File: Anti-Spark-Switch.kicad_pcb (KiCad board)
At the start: 2 copper layers, 63.2 x 30 mm, 40 parts, among them P2 Pad_Conn, P5 Pad_Conn, P6 Pad_Conn, P7 CONN_01X04, Q1 IRFS7530, Q2 IRFS7530, Q3 IRFS7530

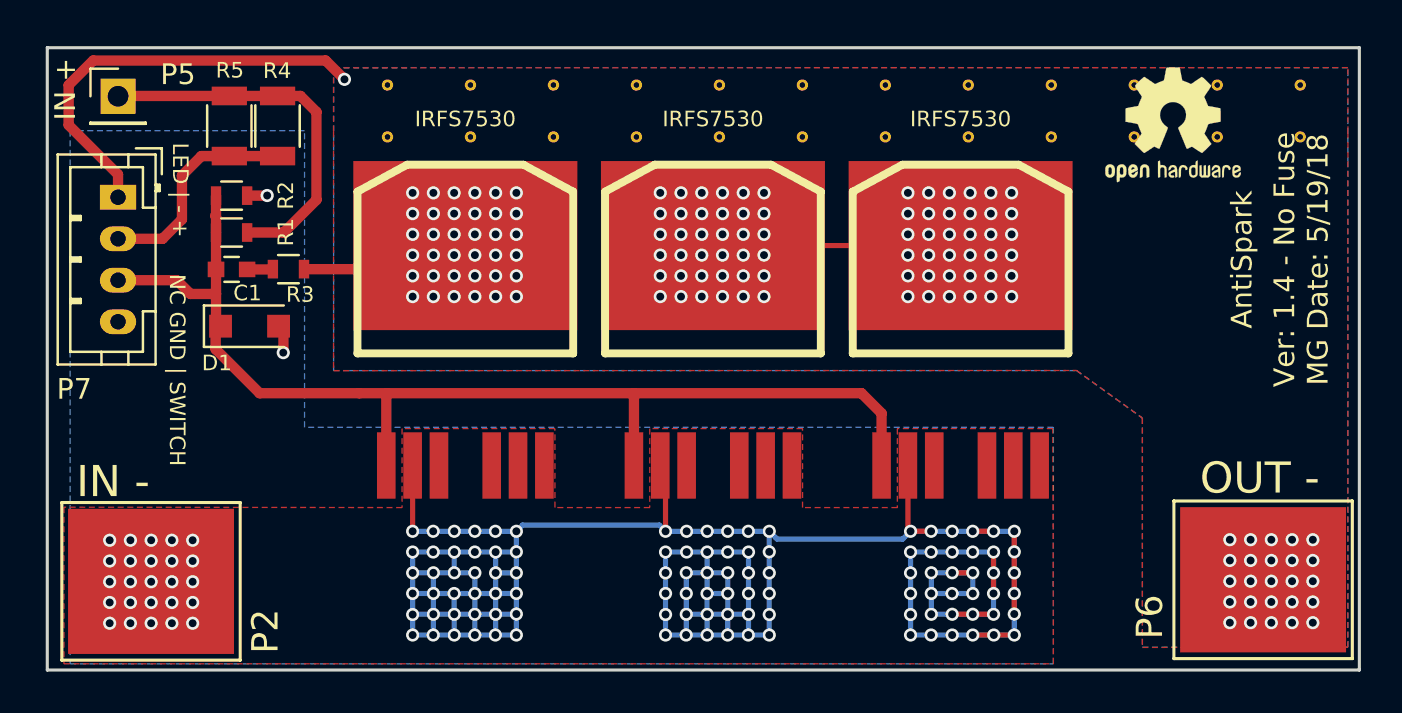
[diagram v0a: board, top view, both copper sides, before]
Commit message: smaller design
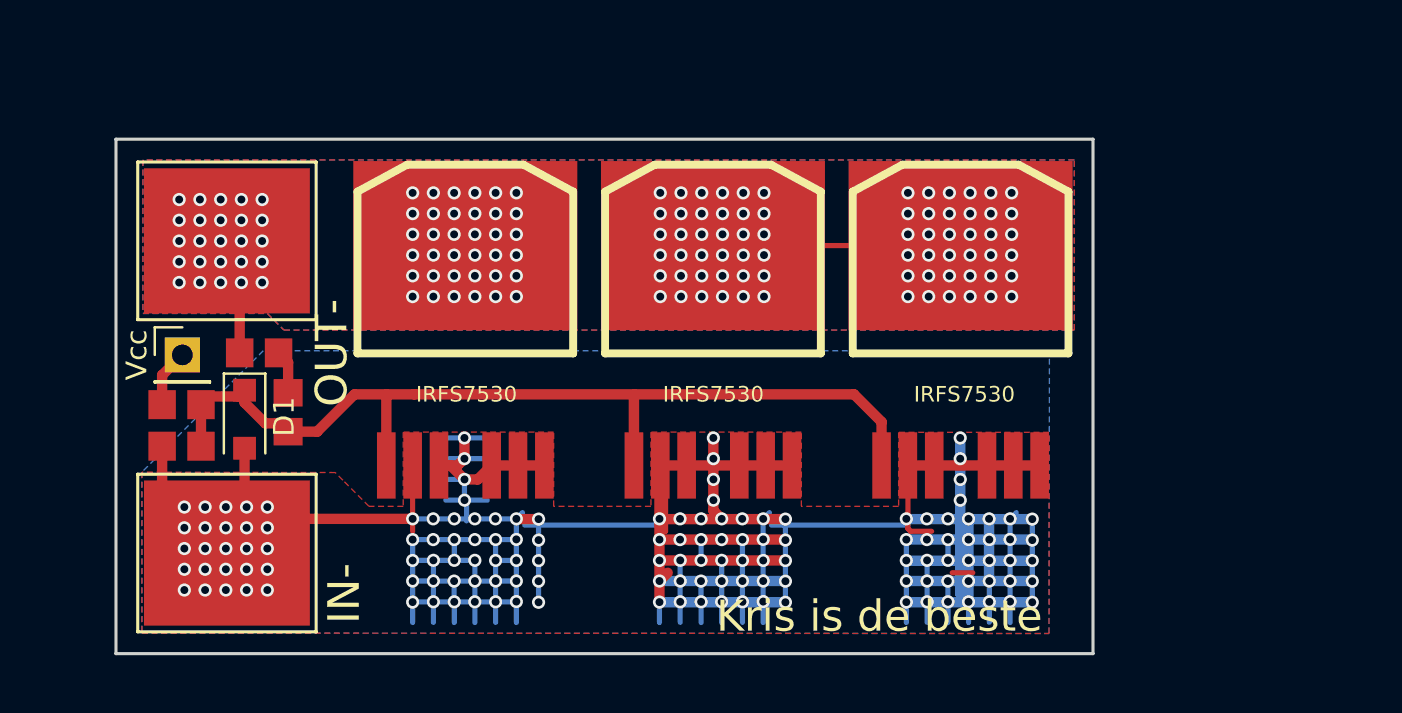
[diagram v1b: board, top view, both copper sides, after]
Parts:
- removed ? (x24): , Kinetic_Footprints:via-0.45mm
- removed C1: 1uF, Capacitors_SMD:C_0603
- removed G***: LOGO, w_logo:Logo_silk_high_voltage_10x8.5mm
- removed P5: Pad_Conn, Connector_PinHeader_2.54mm:PinHeader_1x01_P2.54mm_Vertical
- removed P6: Pad_Conn, sparkparts:1PAD_8x7mm
- removed P7: CONN_01X04, Connector_JST:JST_PH_B4B-PH-K_1x04_P2.00mm_Vertical
- removed R4, R5: 16.5K, Resistors_SMD:R_1206
- removed REF***: OSHW-Logo2_7.3x6mm_SilkScreen, Symbols:OSHW-Logo2_7.3x6mm_SilkScreen
- added 1uF: 1uF, Capacitor_SMD:C_0805_2012Metric_Pad1.33x1.40mm_HandSolder, F.Cu at (127.3, 106.4)
- added OUT-: Pad_Conn, sparkparts:1PAD_8x7mm, F.Cu at (124.3, 98.1)
- added Vcc: VCC NO, Connector_PinHeader_2.54mm:PinHeader_1x01_P2.54mm_Vertical, F.Cu at (122.2, 103.6)
- D1: footprint Diodes_SMD:D_SOD-123F -> Diode_SMD:D_SOD-123F
- R1, R2, R3: footprint Resistors_SMD:R_0603 -> Resistor_SMD:R_0805_2012Metric_Pad1.33x1.40mm_HandSolder
- moved R2 12.3 mm to (122.2, 108.0), turned to 180 degrees
- moved R1 8.64 mm to (122.2, 106.0), turned to 0 degrees
- moved D1 4.49 mm to (125.2, 106.7), turned to 270 degrees
- moved R3 4.28 mm to (125.9, 103.5), turned to 0 degrees
- moved IN- 3.91 mm to (124.3, 113.2)
- renumbered P2 to IN-
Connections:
- net /SW_NC renamed Net-(C1-Pad2)
- R1 pad 1: VCC -> Net-(P5-Pad1)
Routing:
- net GND: track 201.5 -> 357.6 mm, vias 135 -> 142
- net Net-(P6-Pad1): track 116.3 -> 97.5 mm, vias 134 -> 133
- net VCC: track 18.1 -> 0.00 mm
- net Net-(P7-Pad2): track 10.6 -> 0.00 mm
- net Net-(C1-Pad2): track 55.4 -> 47.3 mm
- net Net-(P5-Pad1): track 0.00 -> 3.20 mm
- net Net-(C1-Pad1): track 1.25 -> 2.12 mm
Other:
- board size 63.2 x 30 mm -> 47.1 x 24.8 mm
- board text added: "Kris is de beste"
- board text removed: "AntiSpark"
- board text removed: "IN +"
- board text removed: "IN -"
- board text removed: "LED | - +"
- board text removed: "NC GND | SWITCH"
- board text removed: "OUT -"
- board text removed: "Ver: 1.4 - No Fuse MG Date: 5/19/18"
